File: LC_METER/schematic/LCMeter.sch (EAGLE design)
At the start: 212 parts, among them IC1 MEGA8535, IC10 MC34063, IC2 74HC595, IC3 74HC595, IC4 74HC595, IC5 74HC595, IC6 74HC595, IC7 LM324, IC8 7905, IC9 LM317, J10 0, J100 0, J11 0, J4 0, J6 0, J8 0, Q1 12MHz, T1 BC847, T2 BC857, T3 BC847, T4 BC847, T5 BC847, T6 BC847, T7 BC857, X1 MCU_PROGRAMMING, X2 L_X, X3 C_X, X4 USB_MICRO, X5 USB_B

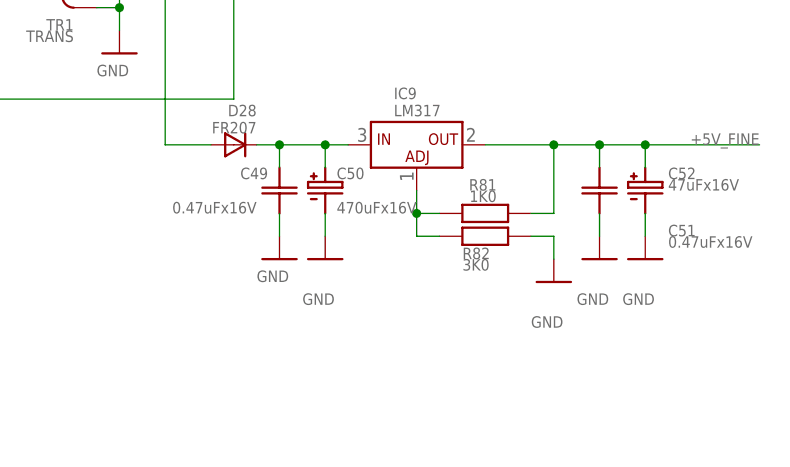
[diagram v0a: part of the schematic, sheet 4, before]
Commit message: LC Metter. Adjust +5v stabilizer values
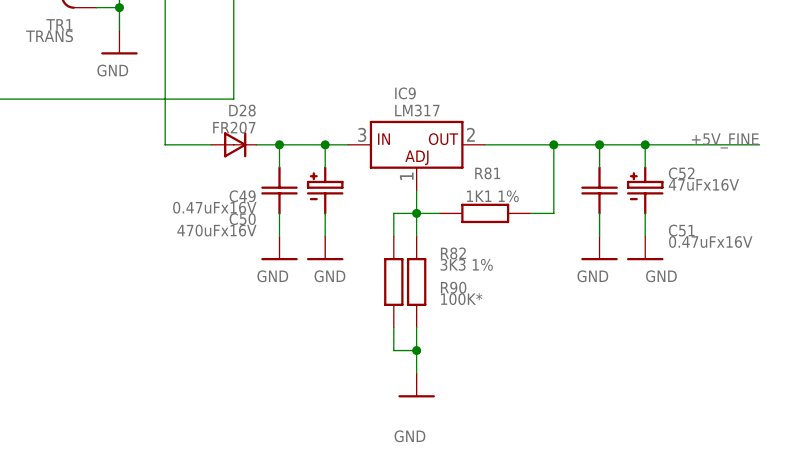
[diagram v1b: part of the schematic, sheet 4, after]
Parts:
- added R90: 100K*, __MyCommonLib1:RSMD_0805
- R81: value 1K0 -> 1K1 1%
- R82: value 3K0 -> 3K3 1%
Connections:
- net GND: now also R90.PIN0
- net N$142: now also R90.PIN1
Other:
- moved on the sheet: R82
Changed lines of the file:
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@@
 <setting verticaltext="up"/>
 </settings>
-<grid distance="0.1" unitdist="inch" unit="inch" style="lines" multiple="1" display="no" altdistance="0.01" altunitdist="inch" altunit="inch"/>
+<grid distance="0.05" unitdist="inch" unit="inch" style="lines" multiple="2" display="yes" altdistance="0.01" altunitdist="inch" altunit="inch"/>
 <layers>
 <layer number="1" name="Top" color="4" fill="1" visible="no" active="no"/>
@@
 <part name="GND79" library="supply1" deviceset="GND" device=""/>
 <part name="GND80" library="supply1" deviceset="GND" device=""/>
-<part name="R81" library="__MyCommonLib1" deviceset="R" device="SMD_0805" value="1K0"/>
-<part name="R82" library="__MyCommonLib1" deviceset="R" device="SMD_0805" value="3K0"/>
+<part name="R81" library="__MyCommonLib1" deviceset="R" device="SMD_0805" value="1K1 1%"/>
+<part name="R82" library="__MyCommonLib1" deviceset="R" device="SMD_0805" value="3K3 1%"/>
 <part name="IC8" library="__MyCommonLib1" deviceset="7905" device="(D2PAK)" value="7905"/>
 <part name="GND82" library="supply1" deviceset="GND" device=""/>
@@
 <part name="GND43" library="supply1" deviceset="GND" device=""/>
 <part name="GND88" library="supply1" deviceset="GND" device=""/>
+<part name="R90" library="__MyCommonLib1" deviceset="R" device="SMD_0805" value="100K*"/>
 </parts>
 <sheets>
@@
 </instance>
 <instance part="C49" gate="C$1" x="177.8" y="66.04" smashed="yes">
-<attribute name="NAME" x="176.53" y="68.58" size="1.27" layer="95" font="vector" ratio="20" rot="R180"/>
+<attribute name="NAME" x="175.26" y="66.04" size="1.27" layer="95" font="vector" ratio="20" rot="R180"/>
 <attribute name="VALUE" x="175.26" y="64.77" size="1.27" layer="96" font="vector" ratio="20" rot="R180"/>
 </instance>
 <instance part="C50" gate="C$1" x="182.88" y="66.04" smashed="yes">
-<attribute name="NAME" x="184.15" y="67.31" size="1.27" layer="95" font="vector" ratio="20"/>
-<attribute name="VALUE" x="184.15" y="63.5" size="1.27" layer="96" font="vector" ratio="20"/>
+<attribute name="NAME" x="175.26" y="63.5" size="1.27" layer="95" font="vector" ratio="20" rot="R180"/>
+<attribute name="VALUE" x="175.26" y="62.23" size="1.27" layer="96" font="vector" ratio="20" rot="R180"/>
 </instance>
 <instance part="GND76" gate="1" x="177.8" y="58.42" smashed="yes">
@@
 </instance>
 <instance part="GND77" gate="1" x="182.88" y="58.42" smashed="yes">
-<attribute name="VALUE" x="180.34" y="53.34" size="1.27" layer="96" font="vector" ratio="20"/>
+<attribute name="VALUE" x="181.61" y="55.88" size="1.27" layer="96" font="vector" ratio="20"/>
 </instance>
 <instance part="IC9" gate="G$1" x="193.04" y="71.12" smashed="yes">
@@
 <attribute name="VALUE" x="190.5" y="74.295" size="1.27" layer="96" font="vector" ratio="20"/>
 </instance>
-<instance part="GND78" gate="1" x="208.28" y="55.88" smashed="yes">
-<attribute name="VALUE" x="205.74" y="50.8" size="1.27" layer="96" font="vector" ratio="20"/>
+<instance part="GND78" gate="1" x="193.04" y="43.18" smashed="yes">
+<attribute name="VALUE" x="190.5" y="38.1" size="1.27" layer="96" font="vector" ratio="20"/>
 </instance>
 <instance part="C51" gate="C$1" x="213.36" y="66.04" smashed="yes">
@@
 </instance>
 <instance part="GND79" gate="1" x="213.36" y="58.42" smashed="yes">
-<attribute name="VALUE" x="210.82" y="53.34" size="1.27" layer="96" font="vector" ratio="20"/>
+<attribute name="VALUE" x="210.82" y="55.88" size="1.27" layer="96" font="vector" ratio="20"/>
 </instance>
 <instance part="GND80" gate="1" x="218.44" y="58.42" smashed="yes">
-<attribute name="VALUE" x="215.9" y="53.34" size="1.27" layer="96" font="vector" ratio="20"/>
+<attribute name="VALUE" x="218.44" y="55.88" size="1.27" layer="96" font="vector" ratio="20"/>
 </instance>
 <instance part="R81" gate="R$1" x="200.66" y="63.5" smashed="yes" rot="R90">
-<attribute name="NAME" x="201.93" y="67.31" size="1.27" layer="95" font="vector" ratio="20" rot="R180"/>
-<attribute name="VALUE" x="201.93" y="66.04" size="1.27" layer="96" font="vector" ratio="20" rot="R180"/>
+<attribute name="NAME" x="199.39" y="67.31" size="1.27" layer="95" font="vector" ratio="20"/>
+<attribute name="VALUE" x="204.47" y="66.04" size="1.27" layer="96" font="vector" ratio="20" rot="R180"/>
 </instance>
-<instance part="R82" gate="R$1" x="200.66" y="60.96" smashed="yes" rot="R90">
-<attribute name="NAME" x="198.12" y="58.42" size="1.27" layer="95" font="vector" ratio="20"/>
-<attribute name="VALUE" x="198.12" y="57.15" size="1.27" layer="96" font="vector" ratio="20"/>
+<instance part="R82" gate="R$1" x="193.04" y="55.88" smashed="yes">
+<attribute name="NAME" x="195.58" y="58.42" size="1.27" layer="95" font="vector" ratio="20"/>
+<attribute name="VALUE" x="195.58" y="57.15" size="1.27" layer="96" font="vector" ratio="20"/>
 </instance>
 <instance part="IC8" gate="G$1" x="182.88" y="149.86" smashed="yes">
@@
 <attribute name="VALUE" x="41.91" y="157.48" size="1.27" layer="96" font="vector" ratio="20" rot="R180"/>
 </instance>
+<instance part="R90" gate="R$1" x="190.5" y="55.88" smashed="yes">
+<attribute name="NAME" x="195.58" y="54.61" size="1.27" layer="95" font="vector" ratio="20"/>
+<attribute name="VALUE" x="195.58" y="53.34" size="1.27" layer="96" font="vector" ratio="20"/>
+</instance>
 </instances>
 <busses>
@@
 <pinref part="R82" gate="R$1" pin="PIN0"/>
 <pinref part="GND78" gate="1" pin="GND"/>
-<wire x1="205.74" y1="60.96" x2="208.28" y2="60.96" width="0.1524" layer="91"/>
-<wire x1="208.28" y1="60.96" x2="208.28" y2="58.42" width="0.1524" layer="91"/>
+<wire x1="193.04" y1="50.8" x2="193.04" y2="48.26" width="0.1524" layer="91"/>
+<pinref part="R90" gate="R$1" pin="PIN0"/>
+<wire x1="193.04" y1="48.26" x2="193.04" y2="45.72" width="0.1524" layer="91"/>
+<wire x1="193.04" y1="48.26" x2="190.5" y2="48.26" width="0.1524" layer="91"/>
+<wire x1="190.5" y1="48.26" x2="190.5" y2="50.8" width="0.1524" layer="91"/>
+<junction x="193.04" y="48.26"/>
 </segment>
 <segment>
@@
 <pinref part="R82" gate="R$1" pin="PIN1"/>
 <pinref part="IC9" gate="G$1" pin="ADJ"/>
-<wire x1="195.58" y1="60.96" x2="193.04" y2="60.96" width="0.1524" layer="91"/>
 <wire x1="193.04" y1="60.96" x2="193.04" y2="63.5" width="0.1524" layer="91"/>
 <pinref part="R81" gate="R$1" pin="PIN1"/>
@@
 <wire x1="195.58" y1="63.5" x2="193.04" y2="63.5" width="0.1524" layer="91"/>
 <junction x="193.04" y="63.5"/>
+<pinref part="R90" gate="R$1" pin="PIN1"/>
+<wire x1="193.04" y1="63.5" x2="190.5" y2="63.5" width="0.1524" layer="91"/>
+<wire x1="190.5" y1="63.5" x2="190.5" y2="60.96" width="0.1524" layer="91"/>
 </segment>
 </net>
